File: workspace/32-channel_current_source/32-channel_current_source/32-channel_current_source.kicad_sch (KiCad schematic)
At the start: 8 parts, among them J1 Conn_01x01, J2 Conn_01x01, J3 Conn_01x01, J4 Conn_02x05_Odd_Even

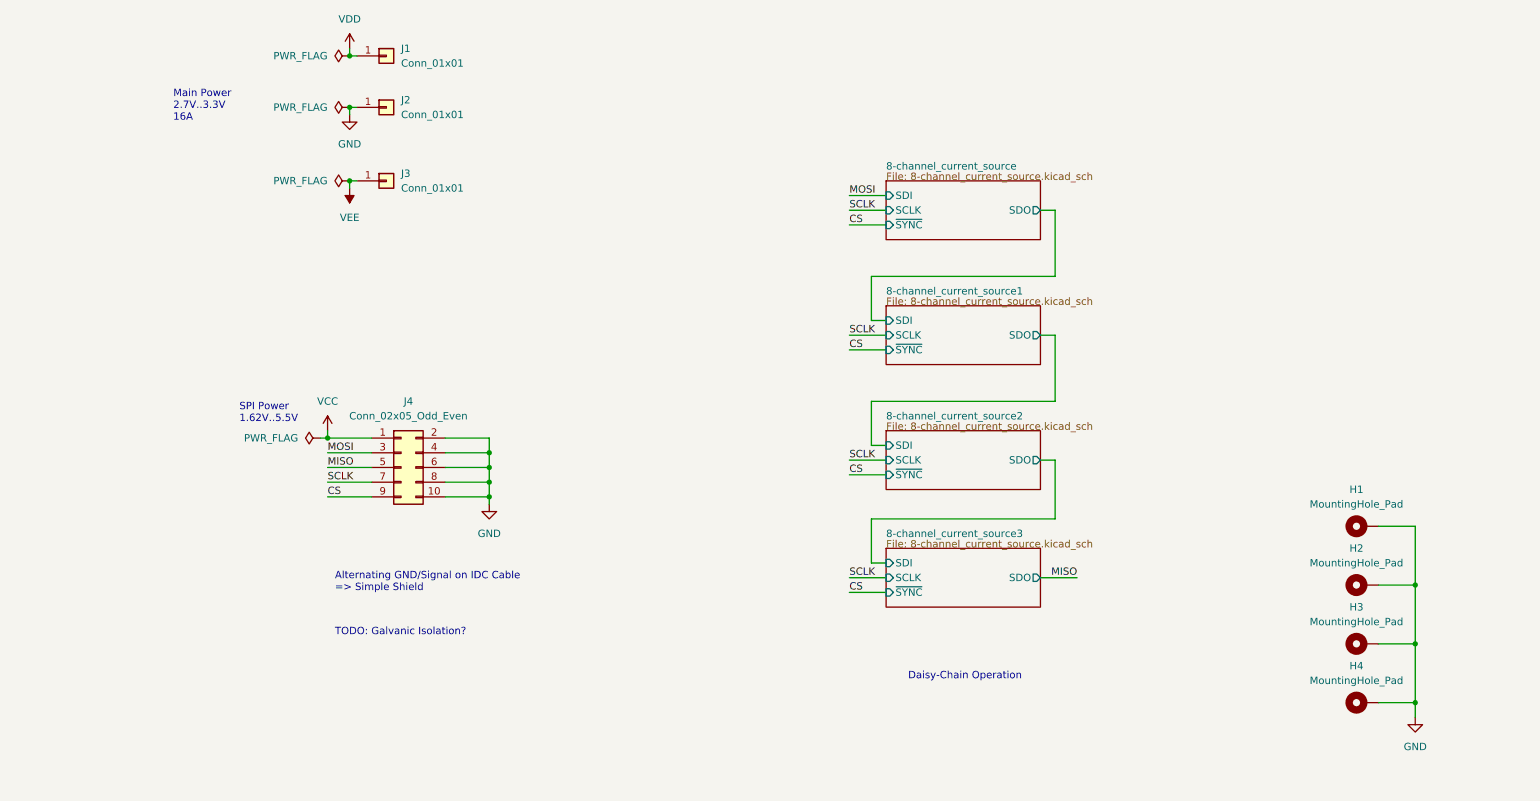
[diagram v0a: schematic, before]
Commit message: Finish Rev 1 of the 32-channel current supply
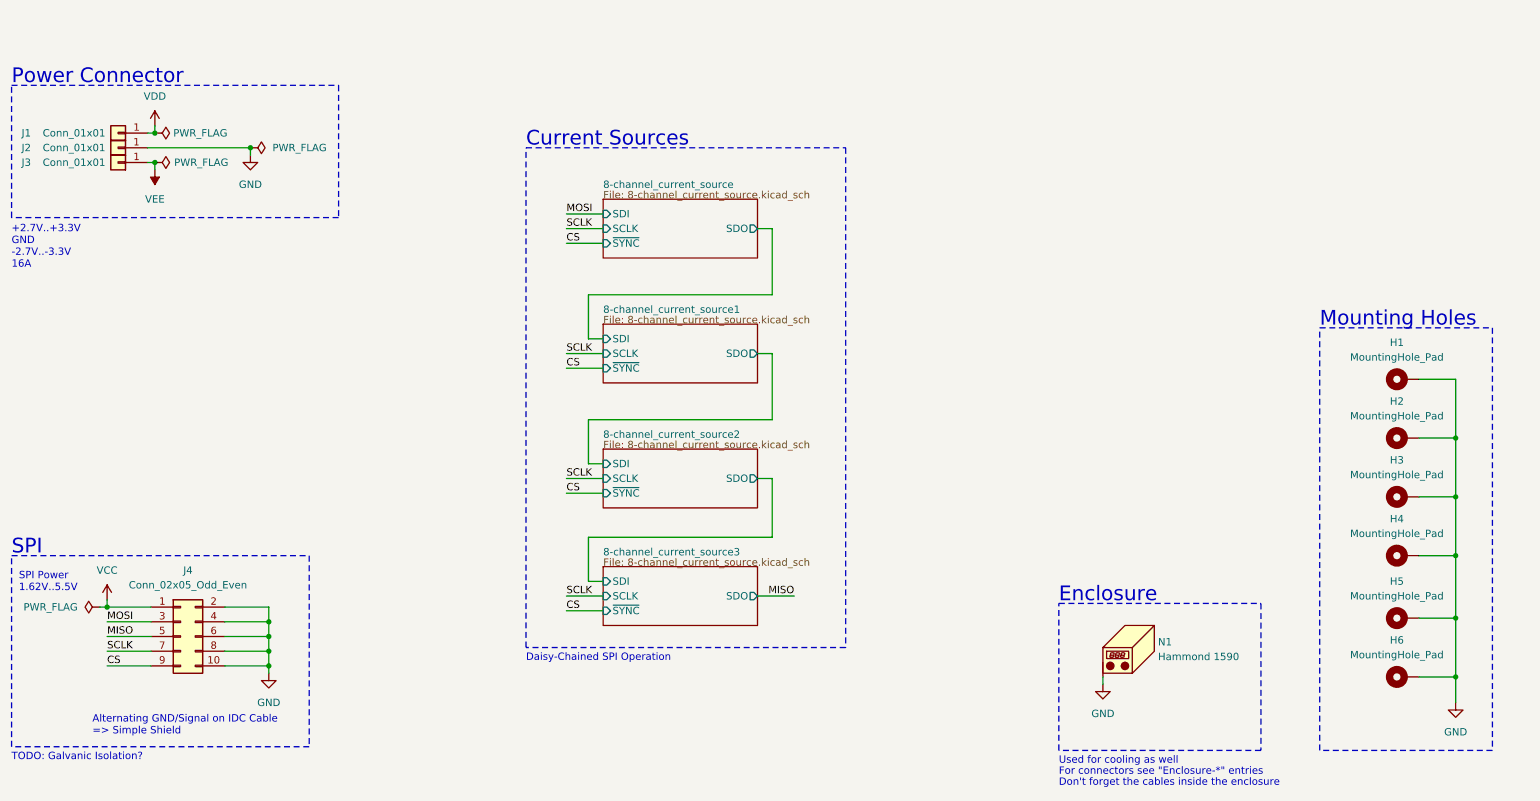
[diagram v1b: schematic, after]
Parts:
- added H5, H6: MountingHole_Pad, MountingHole:MountingHole_6.4mm_M6_ISO14580_Pad, symbol Mechanical:MountingHole_Pad
- added N1: Hammond 1590, symbol Mechanical:Housing_Pad
- H1, H2, H3, H4: footprint MountingHole:MountingHole_3.2mm_M3_Pad_Via -> MountingHole:MountingHole_6.4mm_M6_ISO14580_Pad; now left out of the parts list
- J1: footprint Connector:CalTest_CT3151 -> Connector_Wire:SolderWirePad_1x01_SMD_5x10mm; Enclosure-Datasheet (none) -> https://www.mouser.ch/datasheet/2/215/091-744596.pdf; Enclosure-MPN (none) -> 6091; Enclosure-Mouser (none) -> 534-6091; MPN CT3151-2 -> (none); Mouser 510-CT3151-2 -> (none)
- J2: footprint Connector:CalTest_CT3151 -> Connector_Wire:SolderWirePad_1x01_SMD_5x10mm; Enclosure-Datasheet (none) -> https://www.mouser.ch/datasheet/2/215/092-743448.pdf; Enclosure-MPN (none) -> 6092; Enclosure-Mouser (none) -> 534-6092; MPN CT3151-0 -> (none); Mouser 510-CT3151-0 -> (none)
- J3: footprint Connector:CalTest_CT3151 -> Connector_Wire:SolderWirePad_1x01_SMD_5x10mm; Enclosure-Datasheet (none) -> https://www.mouser.ch/datasheet/2/215/091-744596.pdf; Enclosure-MPN (none) -> 6091; Enclosure-Mouser (none) -> 534-6091; MPN CT3151-0 -> (none); Mouser 510-CT3151-0 -> (none); now left out of the parts list
- J4: Enclosure-Datasheet (none) -> https://www.mouser.ch/datasheet/2/1/7f640c6e18f1d8480b1473b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; Enclosure-MPN (none) -> 4610-6000; Enclosure-Mouser (none) -> 517-4610-6000; MPN (none) -> 72454-010LF; Mouser (none) -> 649-72454-010LF; Notes (none) -> 10 pos, 2 row, DIN41651, 2.54mm PCB pitch, 1.27mm cable pit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; Receptacle-Datasheet (none) -> https://cdn.amphenol-cs.com/media/wysiwyg/files/documentati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; Receptacle-MPN (none) -> 71600-310LF; Receptacle-Mouser (none) -> 649-71600-310LF
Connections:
- net GND: now also H5.1, H6.1, N1.1 (PAD)
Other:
- note added: "+2.7V..+3.3V GND -2.7V..-3.3V 16A"
- note added: "Current Sources"
- note added: "Daisy-Chained SPI Operation"
- note added: "Don't forget the cables inside the enclosure"
- note added: "Enclosure"
- note added: "For connectors see "Enclosure-*" entries"
- note added: "Mounting Holes"
- note added: "Power Connector"
- note added: "SPI"
- note added: "Used for cooling as well"
- note removed: "Daisy-Chain Operation"
- note removed: "Main Power 2.7V..3.3V 16A"
- moved on the sheet: H1, H2, H3, H4, J4
